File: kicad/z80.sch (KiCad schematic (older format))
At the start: 23 parts, among them SW1 SW_PUSH, U1 Z80CPU, U2 z80pcb, U3 74HC14, U4 74LS163

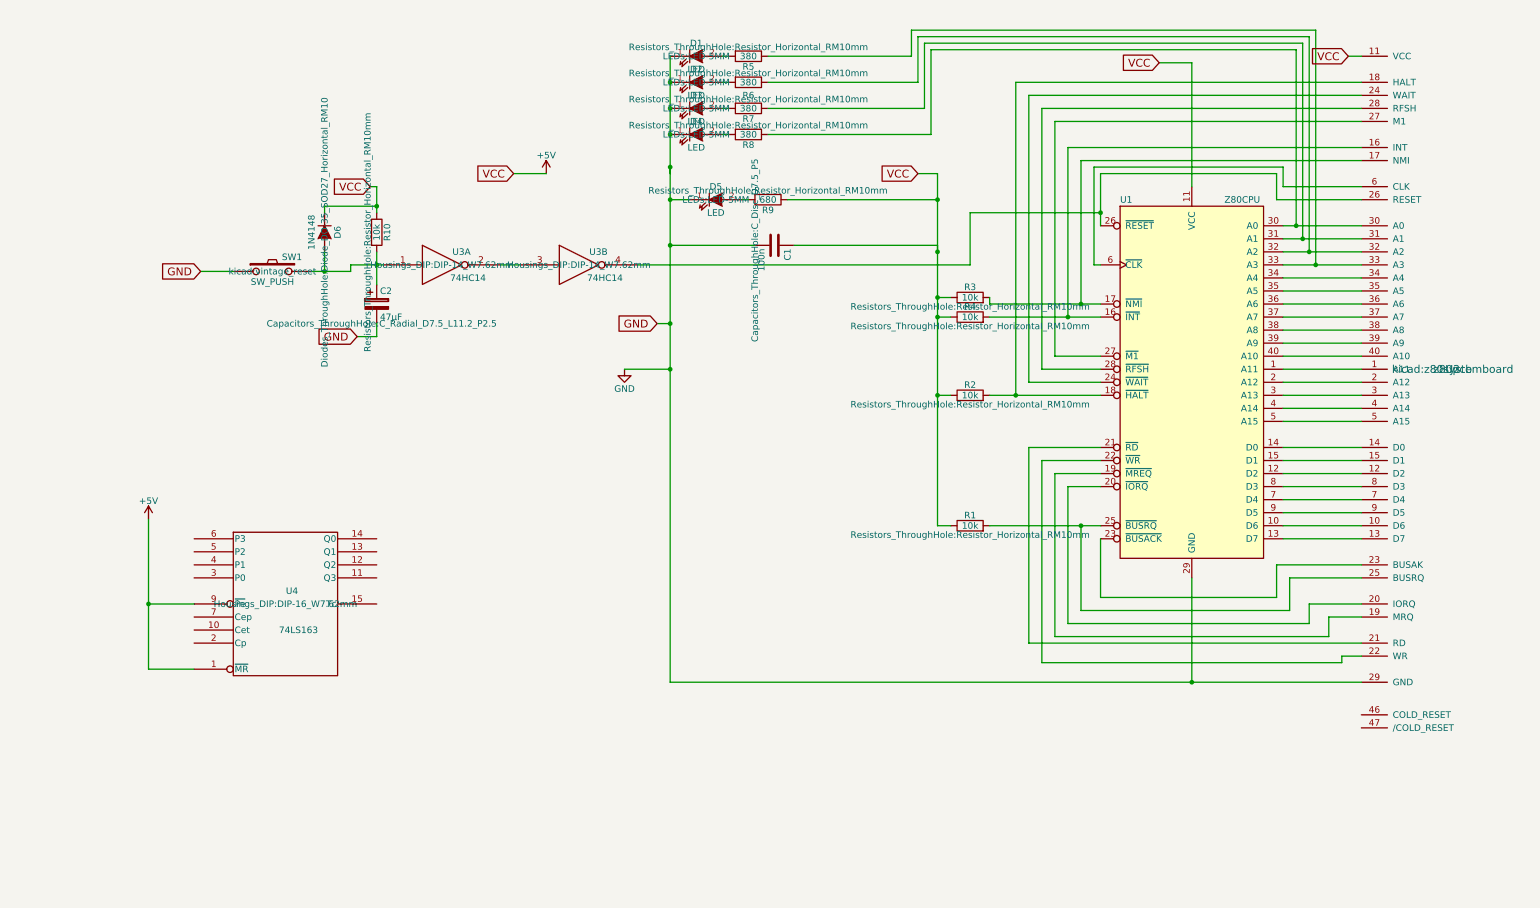
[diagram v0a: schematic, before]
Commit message: finish cpu board draft
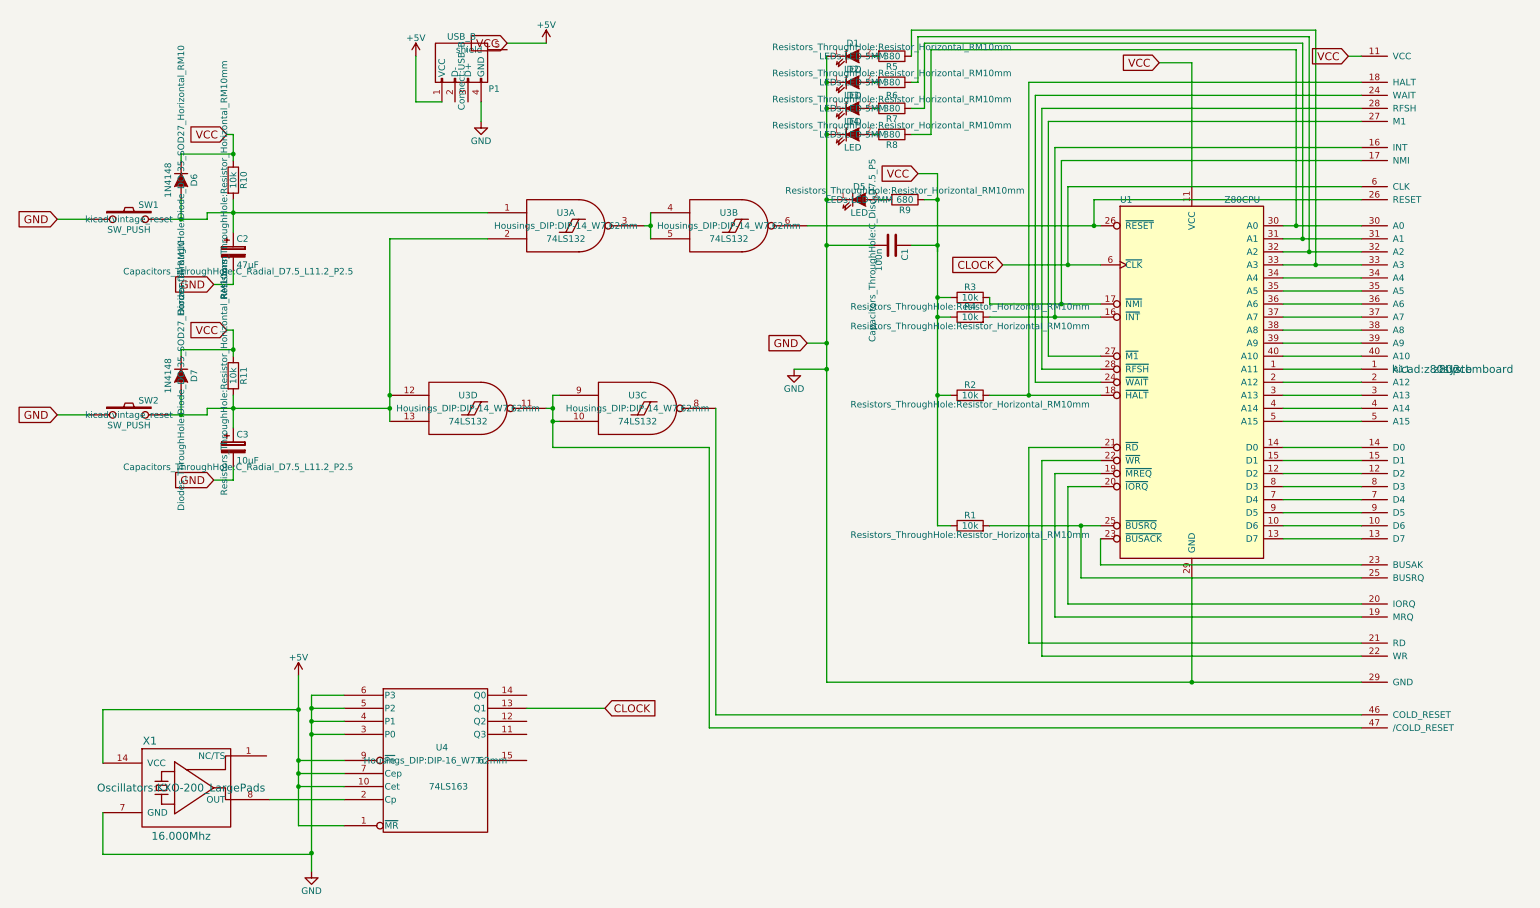
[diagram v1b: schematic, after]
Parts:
- removed U3: 74HC14, Housings_DIP:DIP-14_W7.62mm, symbol 74HC14
- added C3: 10μF, Capacitors_ThroughHole:C_Radial_D7.5_L11.2_P2.5, symbol CP
- added D7: 1N4148, Diodes_ThroughHole:Diode_DO-35_SOD27_Horizontal_RM10, symbol D
- added P1: USB_B, Connect:USB_B, symbol USB_B
- added R11: 10k, Resistors_ThroughHole:Resistor_Horizontal_RM10mm, symbol R
- added SW2: SW_PUSH, kicad:vintage_reset, symbol SW_PUSH
- added U3: 74LS132, Housings_DIP:DIP-14_W7.62mm, symbol 74LS132
- added X1: 16.000Mhz, Oscillators:KXO-200_LargePads, symbol XO-14S
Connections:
- net +5V: now also U4.10 (Cet), U4.7 (Cep), D7.1 (K), P1.1 (VCC), R11.1, U3.14 (VCC), U3.14 (VCC), U3.14 (VCC), U3.14 (VCC), X1.14 (VCC)
- net GND: now also U4.3 (P0), U4.4 (P1), U4.5 (P2), U4.6 (P3), C3.2, P1.4 (GND), SW2.1, U3.7 (GND), U3.7 (GND), U3.7 (GND), U3.7 (GND), X1.7 (GND)
- net at U1.26 (~RESET~), U2.26 (RESET): now also U3.6
- net CLOCK: now reaches U1.6 (~CLK~), U2.6 (CLK)
- net CLOCK: now also U4.13 (Q1)
- net at U2.46 (COLD_RESET): now also U3.8
- net at U2.47 (/COLD_RESET): now also U3.10, U3.11, U3.9
- net at C2.1, D6.2 (A), R10.2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: now also U3.1
- net at U4.2 (Cp): now also X1.8 (OUT)
- new net: C3.1, D7.2 (A), R11.2, SW2.2, U3.12, U3.13, U3.2
- new net: U3.3, U3.4, U3.5
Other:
- moved on the sheet: C1, C2, D1, D2, D3, D4, D5, D6, R10, R5, R6, R7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
